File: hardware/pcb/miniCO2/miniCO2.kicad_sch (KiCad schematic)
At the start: 11 parts, among them J1 USB_A, SW1 SW_Push, U1 ATSAMD21E18A-M, U2 AP2112K-3.3, U3 SCD40-D-R2

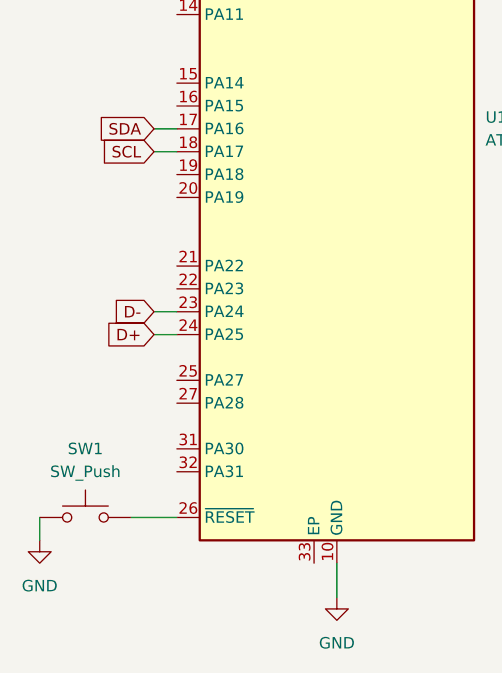
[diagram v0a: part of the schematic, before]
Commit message: Routing finished
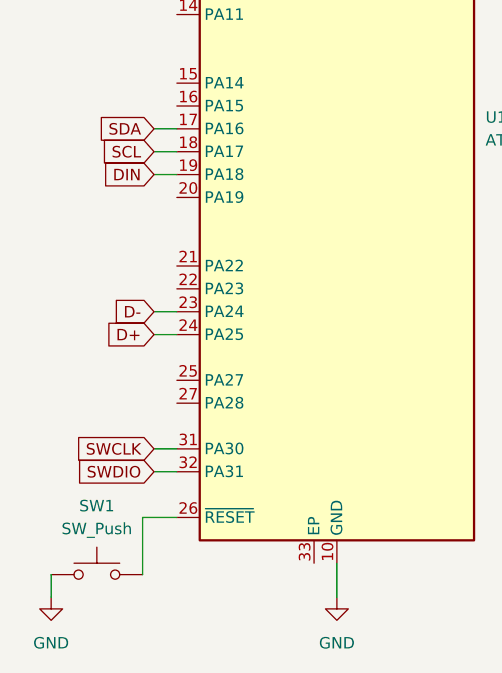
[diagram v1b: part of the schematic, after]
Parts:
- D1, D2: footprint LED_SMD:LED_SK6805_PLCC4_2.4x2.7mm_P1.3mm -> miniCO2:LED_SK6805_PLCC4_2.4x2.7mm_P1.3mm
- U1: footprint Package_DFN_QFN:QFN-32-1EP_5x5mm_P0.5mm_EP3.6x3.6mm -> miniCO2:QFN-32-1EP_5x5mm_P0.5mm_EP3.6x3.6mm
- U3: footprint Sensor:Sensirion_SCD4x-1EP_10.1x10.1mm_P1.25mm_EP4.8x4.8mm -> miniCO2:Sensirion_SCD4x-1EP_10.1x10.1mm_P1.25mm_EP4.8x4.8mm
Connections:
- net DIN: now also U1.19 (PA18)
- net SWCLK: now reaches U1.31 (PA30)
- net SWDIO: now reaches U1.32 (PA31)
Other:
- moved on the sheet: SW1
